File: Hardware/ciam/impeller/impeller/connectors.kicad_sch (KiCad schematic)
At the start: 35 parts, among them J12 Micro-Fit_2x2P, J14 PLS-5, J16 Conn_02x05_SWD, J3 USB_B_Micro, J4 Micro_SD_Card_Con, Q1 BSS138, Q2 BSS138, U4 B0505MT-1WR4, U4 USBLC6-2SC6, U46 HCPL-0630, U47 LDL1117S33R

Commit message: added rpi shield project
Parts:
- C23: Ссылка (none) -> https://www.chipdip.ru/product/grm188r71h104k
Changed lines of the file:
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@@
+      (effects (font (size 1.27 1.27)) hide)
+    )
+    (property "Ссылка" "https://www.chipdip.ru/product/grm188r71h104k" (at 220.98 67.31 0)
       (effects (font (size 1.27 1.27)) hide)
     )

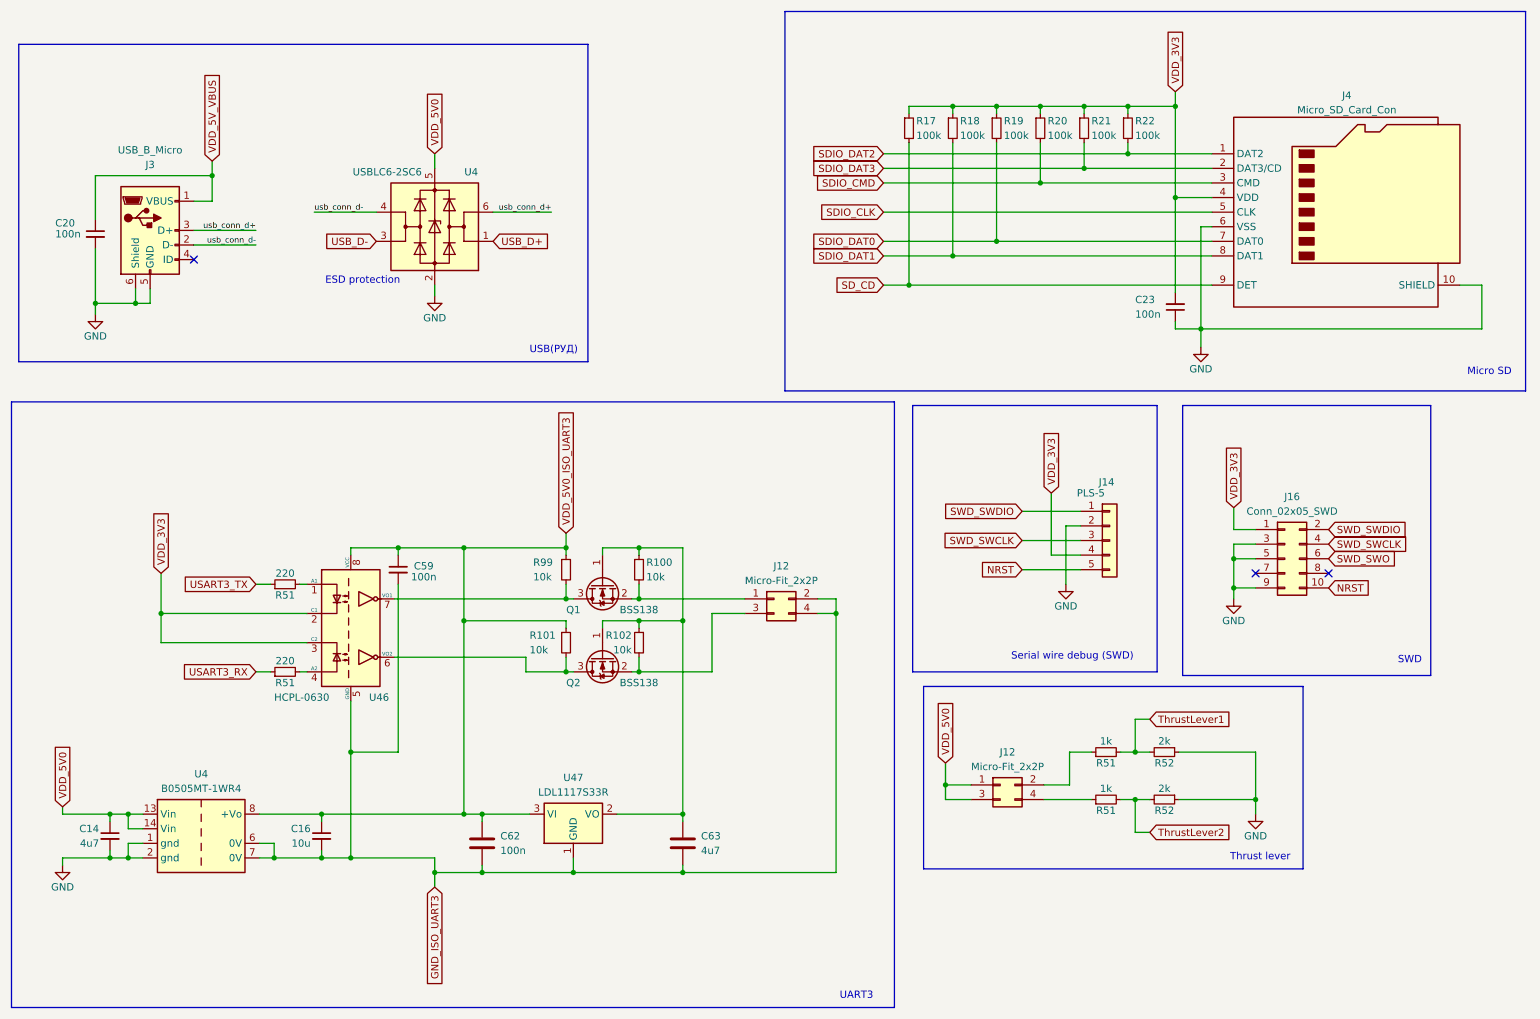
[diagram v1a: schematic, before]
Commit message: fixed uart
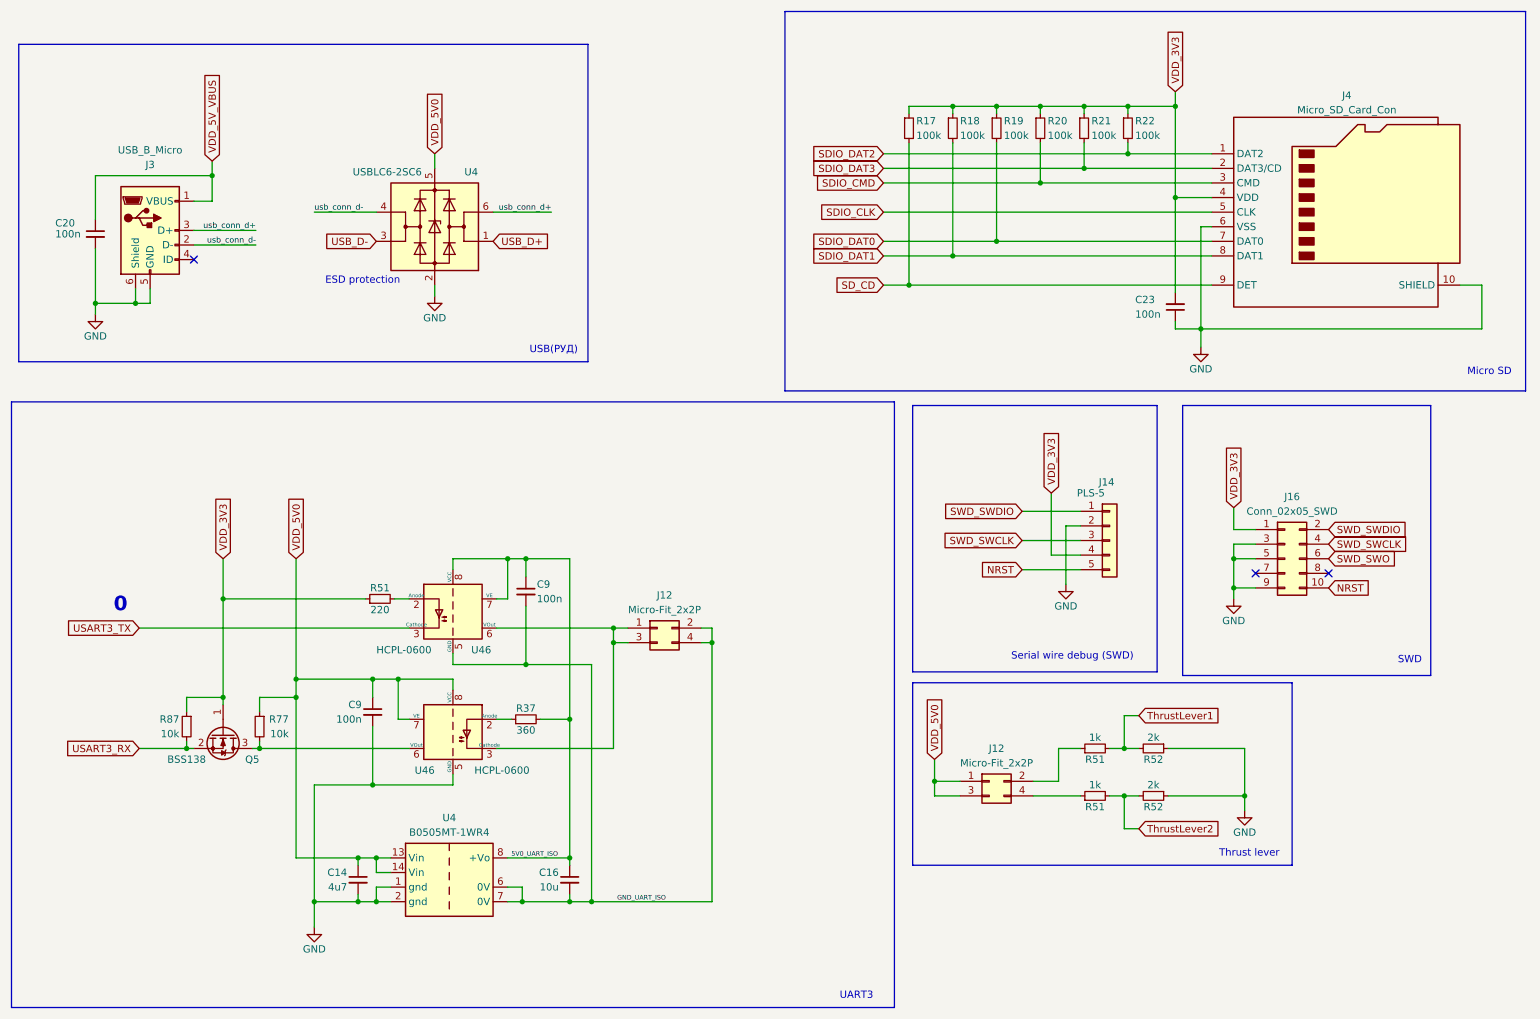
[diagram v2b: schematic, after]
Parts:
- removed C59: 100n, Capacitor_SMD:C_0805_2012Metric, symbol Device:C_Small
- removed C62: 100n, Capacitor_SMD:C_0805_2012Metric, symbol Device:C
- removed C63: 4u7, Capacitor_SMD:C_0805_2012Metric, symbol Device:C
- removed Q1, Q2: BSS138, Package_TO_SOT_SMD:SOT-23, symbol Transistor_FET:BSS138
- removed R100, R101, R102, R99: 10k, Resistor_SMD:R_0805_2012Metric, symbol Device:R_Small
- removed R51 (x2): 220, Resistor_SMD:R_0603_1608Metric, symbol Device:R_Small
- removed U46: HCPL-0630, Package_SO:SOIC-8_3.9x4.9mm_P1.27mm, symbol Isolator:HCPL-0630
- removed U47: LDL1117S33R, Package_TO_SOT_SMD:SOT-223-3_TabPin2, symbol Regulator_Linear:LD1117S33TR_SOT223
- added C9 (x2): 100n, Capacitor_SMD:C_0805_2012Metric, symbol Device:C_Small
- added Q5: BSS138, Package_TO_SOT_SMD:SOT-23, symbol Transistor_FET:BSS138
- added R37: 360, Resistor_SMD:R_0603_1608Metric, symbol Device:R_Small
- added R51: 220, Resistor_SMD:R_0603_1608Metric, symbol Device:R_Small
- added R77, R87: 10k, Resistor_SMD:R_0805_2012Metric, symbol Device:R_Small
- added U46 (x2): HCPL-0600, Package_SO:SO-8_3.9x4.9mm_P1.27mm, symbol Isolator:HCPL-0630
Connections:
- net GND: now also C9.2, U46.5 (GND)
- net USART3_RX: now also Q5.2 (S), R87.2
- net USART3_TX: now also U46.3 (Cathode)
- net VDD_3V3: now also Q5.1 (G), R51.1, R87.1
- net VDD_5V0: now also C9.1, R77.1, U46.7 (VE), U46.8 (VCC)
- net at J12.3 (Pin_3): now also J12.1 (Pin_1), U46.3 (Cathode), U46.6 (VOut)
- net GND_ISO_UART3 renamed GND_UART_ISO
- net GND_UART_ISO: now also C9.2, U46.5 (GND)
- net VDD_5V0_ISO_UART3 renamed 5V0_UART_ISO
- net 5V0_UART_ISO: now also C9.1, R37.2, U46.7 (VE), U46.8 (VCC)
- new net: R37.1, U46.2 (Anode)
- new net: Q5.3 (D), R77.2, U46.6 (VOut)
- new net: R51.2, U46.2 (Anode)
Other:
- note added: "0"
- moved on the sheet: C14, C16, J12, R51, R52, U4
